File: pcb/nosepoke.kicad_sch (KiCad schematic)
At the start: 10 parts, among them J1 0855135013, Q1 PT26-21C/TR8

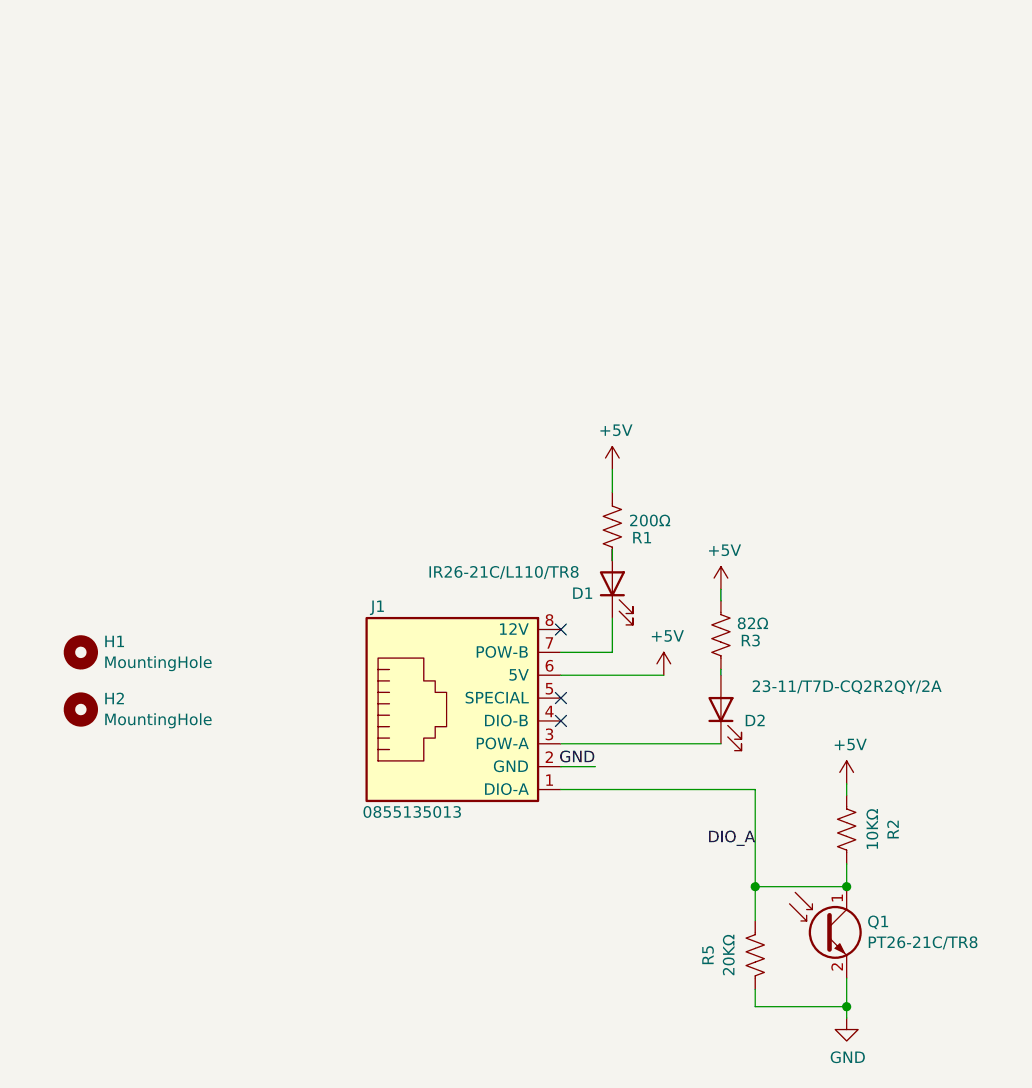
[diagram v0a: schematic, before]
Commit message: backside PCB v1.17
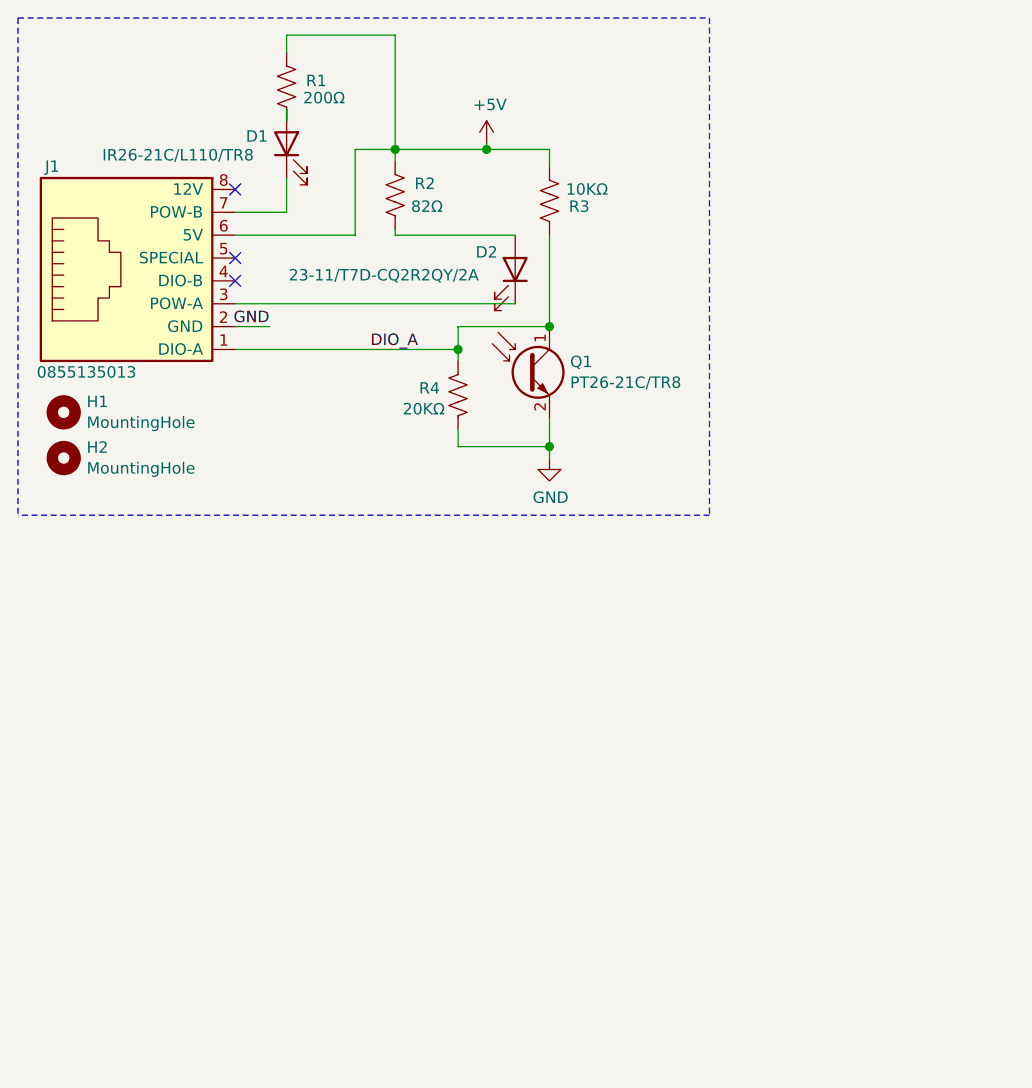
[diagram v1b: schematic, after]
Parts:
- renumbered R3 to R2, R2 to R3, R5 to R4
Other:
- company: (none) -> Andy Lustig
- title: (none) -> Nosepoke
- moved on the sheet: D1, D2, H1, H2, J1, Q1, R1, R2, R3, R4
